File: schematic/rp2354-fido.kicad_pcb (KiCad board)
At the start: 2 copper layers, 18 x 37.5 mm, 36 parts, among them J1 USB_C_Receptacle_USB2.0_14P, SW1 SW_Push, U1 RP2354A, U2 AP2112K-3.3, U3 USBLC6-2SC6, Y1 Crystal_Small

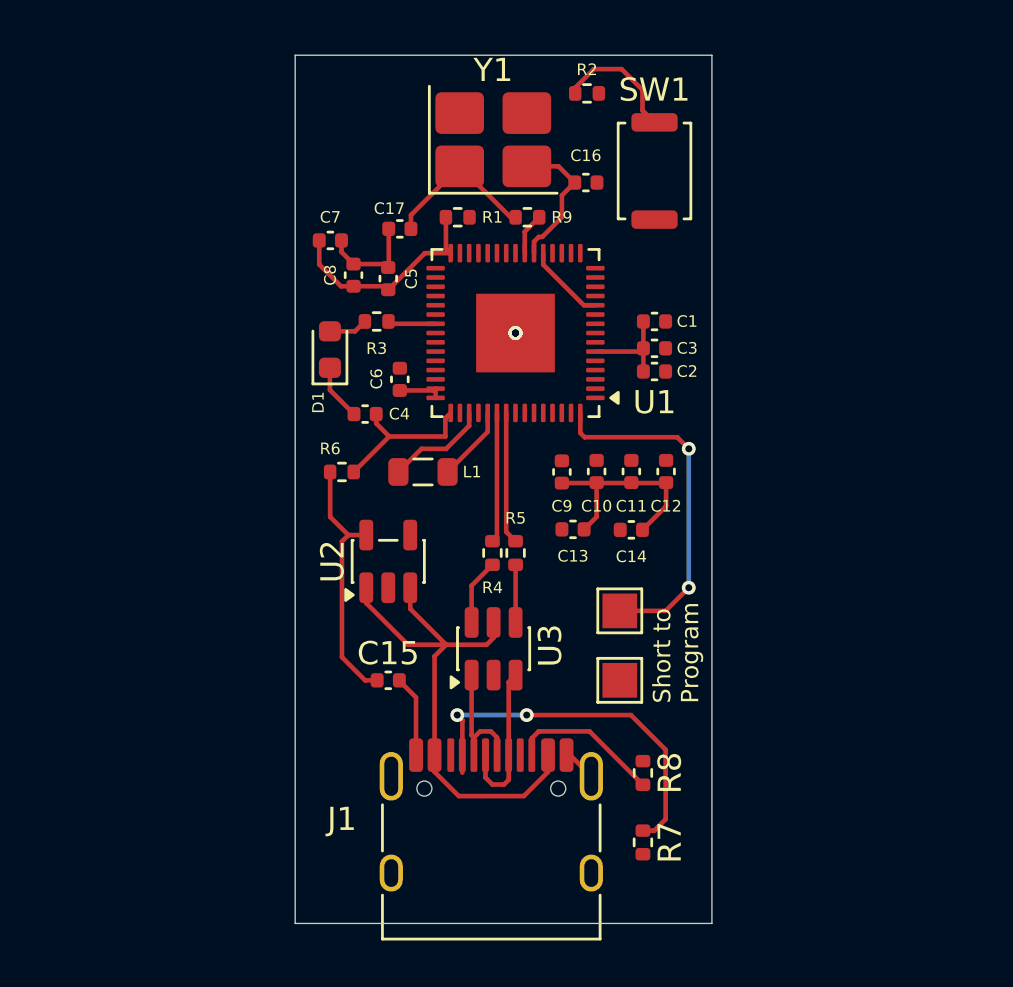
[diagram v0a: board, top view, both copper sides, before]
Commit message: add code, finalize pcb
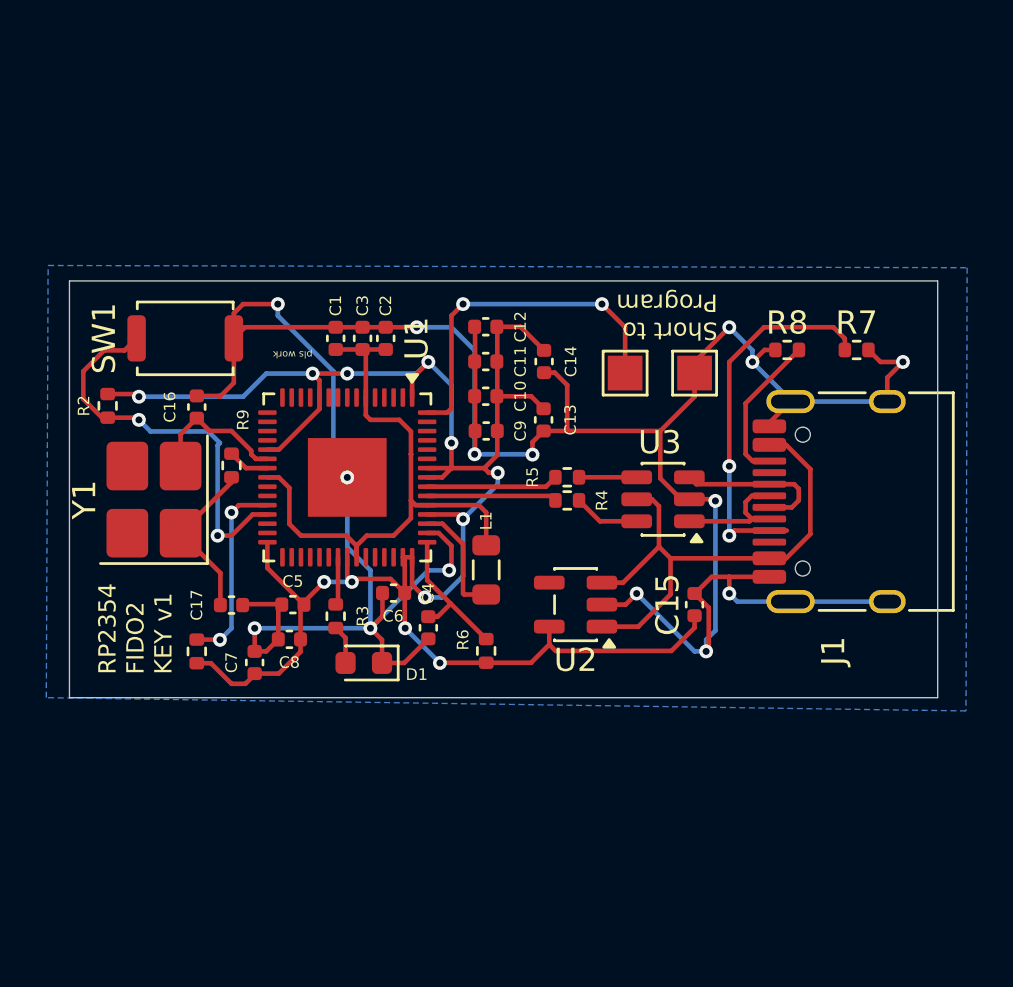
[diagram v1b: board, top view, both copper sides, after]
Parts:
- moved R2 24.7 mm to (94.9, 79.6), turned to -90 degrees
- moved R7 23.2 mm to (127.2, 77.2), turned to 0 degrees
- moved J1 22.0 mm to (127.5, 83.8), turned to 90 degrees
- moved R1 21.9 mm to (98.8, 90.2), turned to -90 degrees
- moved SW1 21.5 mm to (98.2, 76.7), turned to 180 degrees
- moved Y1 21.4 mm to (96.9, 83.7), turned to 90 degrees
- moved C16 19.4 mm to (98.8, 79.7), turned to 90 degrees
- moved R8 19.3 mm to (124.2, 77.2), turned to 0 degrees
- moved C7 18.5 mm to (101.2, 90.7), turned to 90 degrees
- moved C17 17.8 mm to (100.2, 88.2), turned to 180 degrees
- moved R9 16.7 mm to (100.2, 82.2), turned to -90 degrees
- moved C8 16.0 mm to (102.8, 89.7), turned to 180 degrees
- moved C5 14.7 mm to (102.9, 88.2), turned to 0 degrees
- moved C1 13.8 mm to (104.8, 76.7), turned to 90 degrees
- moved TP2 13.7 mm to (120.2, 78.2), turned to 0 degrees
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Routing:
- net GND: track 11.9 -> 130.2 mm, vias 3 -> 15
- net +3V3: track 35.3 -> 88.0 mm, vias 0 -> 12
- net +1V1: track 7.56 -> 25.8 mm
- net Net-(U1-GPIO16): track 5.47 -> 17.3 mm, vias 0 -> 2
- net Net-(U1-RUN): track 0.00 -> 8.39 mm, vias 0 -> 2
- net Net-(U1-VREG_LX): track 4.44 -> 5.06 mm
- added copper zone on B.Cu, net GND
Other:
- board size 18 x 37.5 mm -> 37.5 x 18 mm
- board text added: "RP2354 FIDO2 KEY v1"
- board text added: "pls work"
